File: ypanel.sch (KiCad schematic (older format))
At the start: 58 parts, among them IC2 TSL2561, J1 XF2M-1015-1A, J2 Conn_Coaxial, J3 BATTERY CONNECTOR, J4 B2B-PH-SM4-TB_LF__SN_, U2 Value, U3 SW_SPDT, U4 SW_SPDT

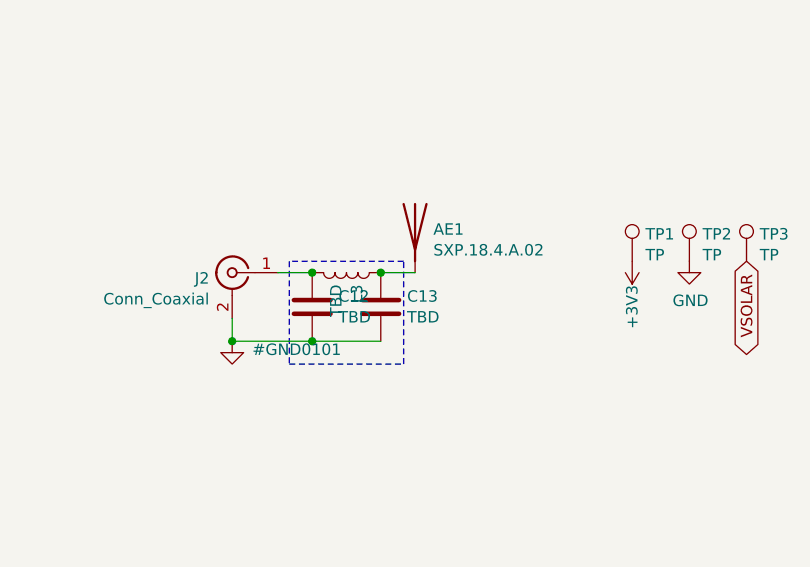
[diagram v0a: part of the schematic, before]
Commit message: clean up & manufacturing output for v3
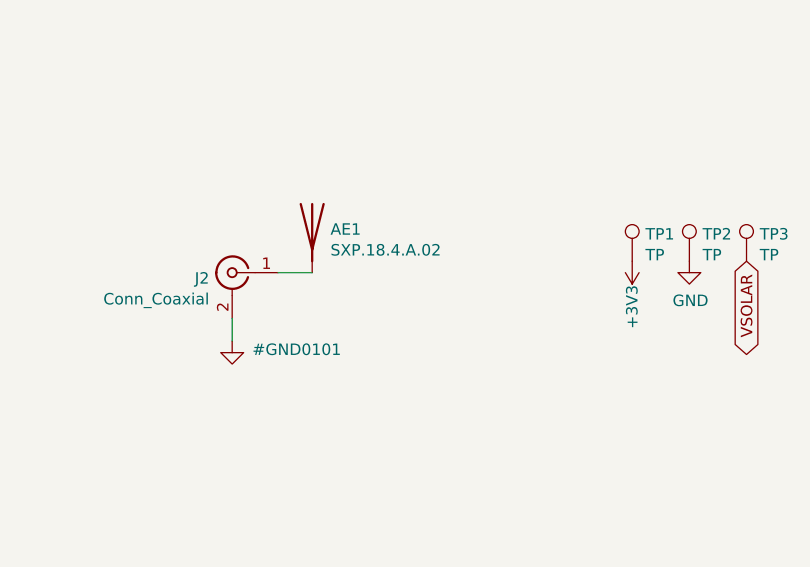
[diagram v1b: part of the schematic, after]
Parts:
- removed C12, C13: TBD, Capacitor_SMD:C_0201_0603Metric, symbol Device:C
- removed L3: TBD, Inductor_SMD:L_0201_0603Metric, symbol Device:L
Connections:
- net at AE1.1 (A): now also J2.1 (In)
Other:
- moved on the sheet: AE1
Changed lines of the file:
@@
 EESchema Schematic File Version 4
-LIBS:ypanel-cache
-EELAYER 26 0
+EELAYER 30 0
 EELAYER END
 $Descr A3 16535 11693
@@
 	1840 8150 1850 8150
 $Comp
-L Device:Antenna AE1
-U 1 1 5E47036D
-P 8350 8300
-F 0 "AE1" H 8430 8289 50  0000 L CNN
-F 1 "SXP.18.4.A.02" H 8430 8198 50  0000 L CNN
-F 2 "spacecraft-footprints:SXP.18.4.A.02" H 8350 8300 50  0001 C CNN
-F 3 "~" H 8350 8300 50  0001 C CNN
-	1    8350 8300
-	1    0    0    -1
-$EndComp
-$Comp
-L Device:L L3
-U 1 1 5E48B702
-P 8050 8500
-F 0 "L3" H 8102 8546 50  0000 L CNN
-F 1 "TBD" H 8102 8455 50  0000 L CNN
-F 2 "Inductor_SMD:L_0201_0603Metric" H 8050 8500 50  0001 C CNN
-F 3 "~" H 8050 8500 50  0001 C CNN
-	1    8050 8500
-	0    1    1    0
-$EndComp
-$Comp
-L Device:C C12
-U 1 1 5E48D592
-P 7900 8650
-F 0 "C12" H 8015 8696 50  0000 L CNN
-F 1 "TBD" H 8015 8605 50  0000 L CNN
-F 2 "Capacitor_SMD:C_0201_0603Metric" H 7938 8500 50  0001 C CNN
-F 3 "~" H 7900 8650 50  0001 C CNN
-	1    7900 8650
-	1    0    0    -1
-$EndComp
-$Comp
-L Device:C C13
-U 1 1 5E48F12E
-P 8200 8650
-F 0 "C13" H 8315 8696 50  0000 L CNN
-F 1 "TBD" H 8315 8605 50  0000 L CNN
-F 2 "Capacitor_SMD:C_0201_0603Metric" H 8238 8500 50  0001 C CNN
-F 3 "~" H 8200 8650 50  0001 C CNN
-	1    8200 8650
-	1    0    0    -1
-$EndComp
-$Comp
 L Connector:Conn_Coaxial J2
 U 1 1 5E49C20B
@@
 	-1   0    0    -1
 $EndComp
-Wire Wire Line
-	8200 8500 8350 8500
-Wire Wire Line
-	7750 8500 7900 8500
-Connection ~ 7900 8500
-Wire Wire Line
-	8200 8800 7900 8800
 $Comp
 L ypanel-rescue:GND-power #GND0101
@@
 	7550 8700 7550 8800
 Wire Wire Line
-	7900 8800 7550 8800
-Connection ~ 7900 8800
-Connection ~ 7550 8800
-Wire Notes Line
-	7800 8450 7800 8900
-Wire Notes Line
-	7800 8900 8300 8900
-Wire Notes Line
-	8300 8900 8300 8450
-Wire Notes Line
-	8300 8450 7800 8450
-Connection ~ 8200 8500
+	7750 8500 7900 8500
+$Comp
+L Device:Antenna AE1
+U 1 1 5E47036D
+P 7900 8300
+F 0 "AE1" H 7980 8289 50  0000 L CNN
+F 1 "SXP.18.4.A.02" H 7980 8198 50  0000 L CNN
+F 2 "spacecraft-footprints:SXP.18.4.A.02" H 7900 8300 50  0001 C CNN
+F 3 "~" H 7900 8300 50  0001 C CNN
+	1    7900 8300
+	1    0    0    -1
+$EndComp
 $EndSCHEMATC
